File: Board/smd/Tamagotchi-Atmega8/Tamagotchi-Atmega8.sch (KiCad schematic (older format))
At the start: 27 parts, among them J1 Conn_02x05_Odd_Even, J2 Conn_01x02, J3 Conn_01x04, J4 Conn_01x07, J5 Conn_01x02, Q1 Q_NPN_BEC, SW1 SW_Push, U1 AMS1117, U2 ATmega328-AU, U3 DS1307Z+, X1 8MHz, X2 32768kHz

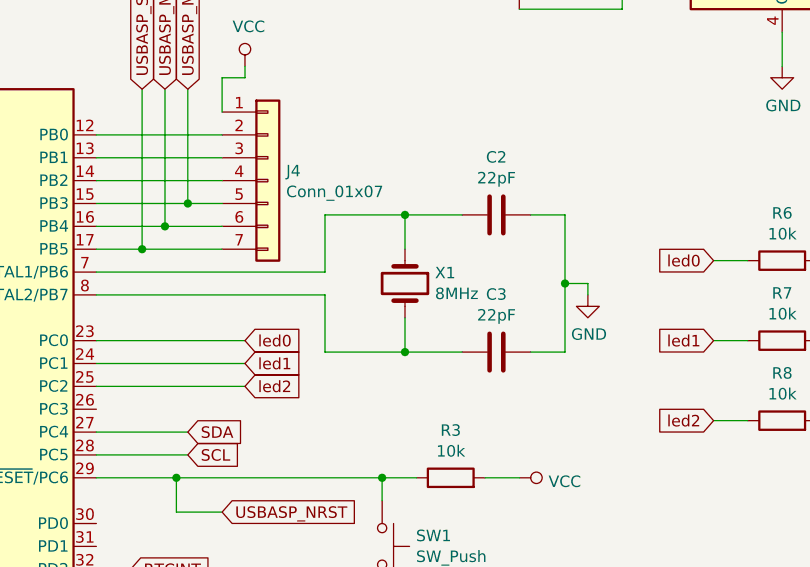
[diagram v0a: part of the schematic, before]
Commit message: Board enhancement
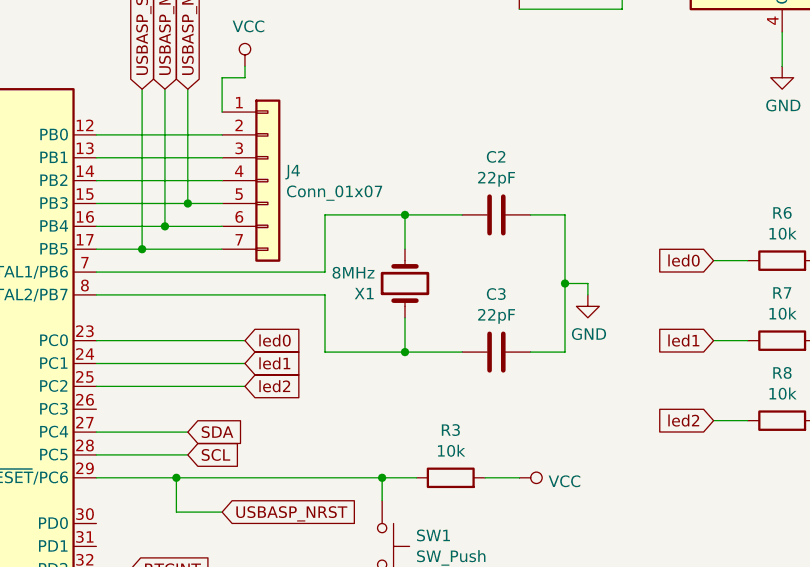
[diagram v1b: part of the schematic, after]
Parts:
- SW1: footprint Button_Switch_SMD:SW_SPST_Panasonic_EVQPL_3PL_5PL_PT_A15 -> Button_Switch_SMD:SW_SPST_B3S-1000
- X1: footprint Crystal:Crystal_SMD_0603-2Pin_6.0x3.5mm_HandSoldering -> Crystal:Crystal_SMD_3225-4Pin_3.2x2.5mm
- X2: footprint Crystal:Crystal_C38-LF_D3.0mm_L8.0mm_Horizontal_1EP_style2 -> Crystal:Crystal_AT310_D3.0mm_L10.0mm_Horizontal_1EP_style2
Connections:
- net at C2.2, U2.7 (XTAL1/PB6): now also X1.2; no longer X1.1
- net at C3.2, U2.8 (XTAL2/PB7): now also X1.1; no longer X1.2
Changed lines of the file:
@@
 F 0 "X2" V 6496 1969 50  0000 R CNN
 F 1 "32768kHz" V 6405 1969 50  0000 R CNN
-F 2 "Crystal:Crystal_C38-LF_D3.0mm_L8.0mm_Horizontal_1EP_style2" H 6450 2100 50  0001 C CNN
+F 2 "Crystal:Crystal_AT310_D3.0mm_L10.0mm_Horizontal_1EP_style2" H 6450 2100 50  0001 C CNN
 F 3 "~" H 6450 2100 50  0001 C CNN
 	1    6450 2100
@@
 F 0 "SW1" V 5804 4748 50  0000 L CNN
 F 1 "SW_Push" V 5895 4748 50  0000 L CNN
-F 2 "Button_Switch_SMD:SW_SPST_Panasonic_EVQPL_3PL_5PL_PT_A15" H 5850 4800 50  0001 C CNN
+F 2 "Button_Switch_SMD:SW_SPST_B3S-1000" H 5850 4800 50  0001 C CNN
 F 3 "~" H 5850 4800 50  0001 C CNN
 	1    5850 4600
@@
 	6200 3150 5950 3150
 Wire Wire Line
-	5950 3150 5950 3300
-Wire Wire Line
-	5950 3600 5950 3750
+	5950 3750 5950 3600
+Wire Wire Line
+	5950 3300 5950 3150
 Wire Wire Line
 	5950 3750 6200 3750
@@
 F 0 "X1" V 5904 3581 50  0000 L CNN
 F 1 "8MHz" V 5995 3581 50  0000 L CNN
-F 2 "Crystal:Crystal_SMD_0603-2Pin_6.0x3.5mm_HandSoldering" H 5950 3450 50  0001 C CNN
+F 2 "Crystal:Crystal_SMD_3225-4Pin_3.2x2.5mm" H 5950 3450 50  0001 C CNN
 F 3 "~" H 5950 3450 50  0001 C CNN
 	1    5950 3450
-	0    1    1    0
+	0    -1   -1   0
 $EndComp
 Text GLabel 4750 4700 2    50   Input ~ 0
@@
 	5250 2550 5250 2500
 $Comp
-L power:VCC #PWR?
+L power:VCC #PWR0101
 U 1 1 5E397814
 P 5250 2500
-F 0 "#PWR?" H 5250 2350 50  0001 C CNN
+F 0 "#PWR0101" H 5250 2350 50  0001 C CNN
 F 1 "VCC" H 5267 2673 50  0000 C CNN
 F 2 "" H 5250 2500 50  0001 C CNN
